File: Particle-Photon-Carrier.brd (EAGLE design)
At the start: 46 x 35.3 mm, 44 parts, among them J2 5V @ 2A, Q1 BSS138, Q2 BSS138, Q3 BSS138, Q4 BSS138

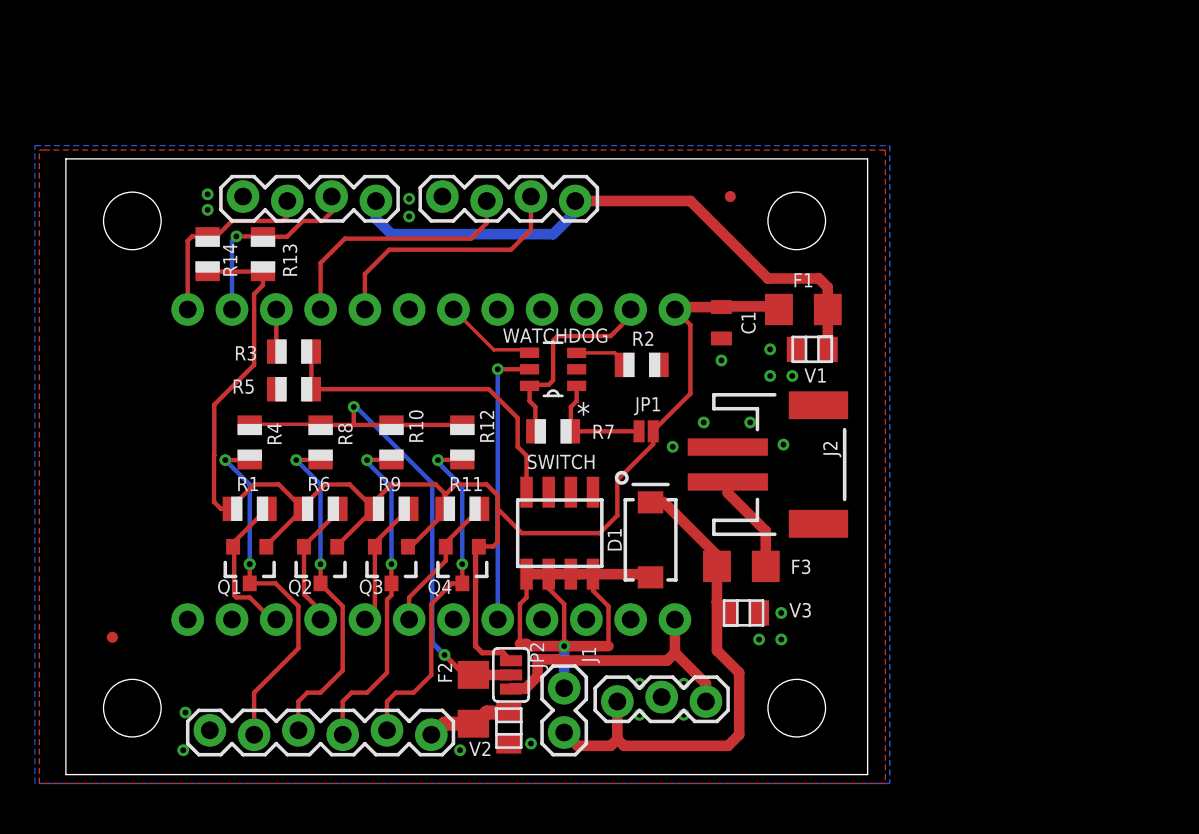
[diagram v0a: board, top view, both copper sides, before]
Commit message: v3 of the AquaMaster
For Spring 2018
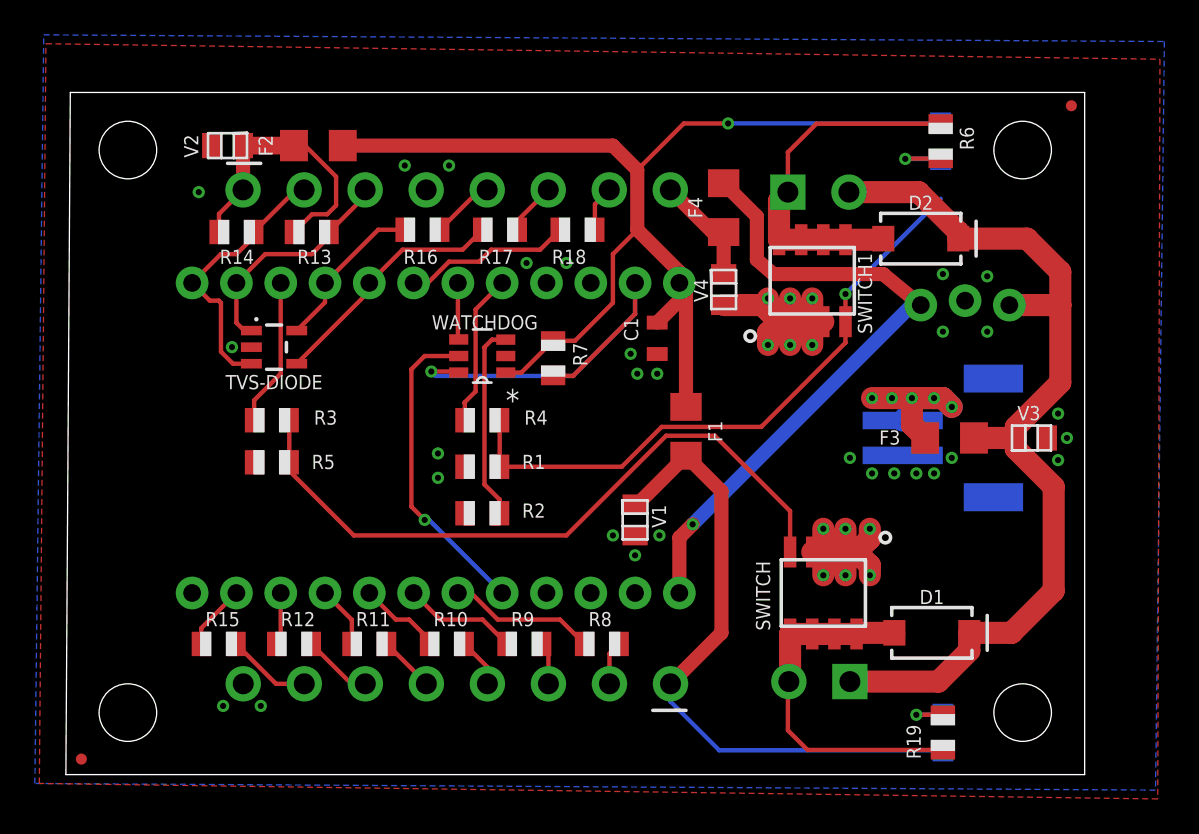
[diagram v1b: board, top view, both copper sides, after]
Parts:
- removed 12V-5V-BUCK: I50115, SparkFun-Connectors:1X03_LOCK
- removed D-IO, I2C: (no value), SparkFun-Connectors:1X04_LOCK
- removed JP1: DOG-SW, SparkFun-Jumpers:SMT-JUMPER_2_NO_NO-SILK
- removed JP2: VSelect, SparkFun-Jumpers:SMT-JUMPER_3_1-NC_PASTE_SILK
- removed Q1, Q2, Q3, Q4: BSS138, SparkFun:SOT23-3
- removed SPI: (no value), SparkFun-Connectors:1X06_LOCK
- added ANALOG, DIGITAL: (no value), SparkFun-Connectors:SCREWTERMINAL-3.5MM-8
- added D2: 3A/40V/500mV, SparkFun-DiscreteSemi:SMA-DIODE
- added F4: 500mA - FAST BLOW, SparkFun-Fuses:1206
- added J3: (no value), SparkFun-Connectors:1X03_LOCK
- added J4: (no value), SparkFun-Connectors:SCREWTERMINAL-3.5MM-2
- added LED1, LED2: (no value), adafruit:CHIPLED_0805
- added R15, R16, R17, R18, R19: 1k, adafruit:R0805
- added SWITCH1: IRF6201PBF, MOSFETs:SO8-GW300
- added TVS-DIODE: D5V0L4B5TS, Custom Components:SOT-23-5
- added V4: VC080505C150DP, Custom Components:0805
- J1: device SparkFun-Connectors:1X02 -> SparkFun-Connectors:SCREWTERMINAL-3.5MM-2
- R1: value 10K -> 100k
- R10, R11, R12, R4, R6, R8, R9: value 10K -> 1k
- moved R6 41.3 mm to (50.2, 36.3), turned to 90 degrees
- moved V2 37.1 mm to (9.27, 36.1), turned to 0 degrees
- moved F2 33.0 mm to (14.5, 36.1), turned to 180 degrees
- moved FD2 20.2 mm to (57.7, 38.4)
- moved R8 19.8 mm to (30.7, 7.49), turned to 0 degrees
- moved V3 19.3 mm to (55.4, 19.3)
- moved D1 17.0 mm to (49.7, 8.13), turned to 0 degrees
- moved J1 16.4 mm to (45.0, 5.33), flipped to the bottom, turned to 0 degrees
- moved SWITCH 15.5 mm to (43.4, 10.4)
- moved R12 15.1 mm to (13.1, 7.49), turned to 0 degrees
- moved V1 14.1 mm to (32.6, 14.6), turned to 90 degrees
- moved F3 14.0 mm to (50.7, 19.3), turned to 0 degrees
- moved JP5 13.6 mm to (54.9, 35.8)
- moved R1 13.6 mm to (23.9, 17.7)
- moved R4 13.4 mm to (23.9, 20.3), turned to 0 degrees
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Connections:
- net SOLENOID renamed SOLENOID1
- removed net A2-EXT: Q1.3, R4.2, SPI.2
- removed net A3-EXT: Q2.3, R8.2, SPI.3
- removed net A4-EXT: Q3.3, R10.2, SPI.4
- removed net A5-EXT: Q4.3, R12.2, SPI.5
- removed net VCC-EXT: D-IO.4, F1.2, I2C.4, V1.2
- removed net VIO-EXT: F2.2, SPI.6, V2.2
- removed net VSELECT: F2.1, JP2.2, R10.1, R12.1, R4.1, R8.1
- new net A0: PHOTON.12
- new net A1: PHOTON.11, R15.1
- new net D5: PHOTON.18, R18.1
- new net DAC: PHOTON.6, R8.1
- new net EXT-A1: ANALOG.7, R15.2
- new net EXT-A2: ANALOG.6, R12.2
- new net EXT-A3: ANALOG.5, R11.2
- new net EXT-A4: ANALOG.4, R10.2
- new net EXT-A5: ANALOG.3, R9.2
- new net EXT-D3: DIGITAL.5, R16.2
- new net EXT-D4: DIGITAL.6, R17.2
- new net EXT-D5: DIGITAL.7, R18.2
- new net EXT-DAC: ANALOG.2, R8.2
- new net GATE1: R1.2, R4.2, SWITCH1.4
- new net LOAD-GND2: D2.A, J4.1, R6.2, SWITCH1.5, SWITCH1.6, SWITCH1.7, SWITCH1.8
- new net N$2: LED1.C, R19.2
- new net RX: PHOTON.4
- new net SOLENOID2: PHOTON.20, R4.1
- new net TX: PHOTON.3
- new net VCC1-EXT: ANALOG.1, F1.2, LED1.A, V1.2
- new net VCC2-EXT: DIGITAL.1, F2.2, R13.2, R14.2, V2.2
- new net VIN-EXT: DIGITAL.8, F4.2, V4.2
- net A2: now also R12.1; no longer Q1.2, R1.2
- net A3: now also R11.1; no longer Q2.2, R6.2
- net A4: now also R10.1; no longer Q3.2, R9.2
- net A5: now also R9.1; no longer Q4.2, R11.2
- net D3: now also R16.1, TVS-DIODE.5; no longer D-IO.2
- net D4: now also R17.1, TVS-DIODE.4; no longer D-IO.3
- net DC-IN: now also D2.C, J1.1, J3.3, J4.2; no longer 12V-5V-BUCK.3, J1.2
- net GND: now also ANALOG.8, DIGITAL.4, J3.2, R1.1, SWITCH1.1, SWITCH1.2, SWITCH1.3, TVS-DIODE.2, V4.1; no longer 12V-5V-BUCK.2, D-IO.1, I2C.1, SPI.1
- net LOAD-GND: now also J1.2, R19.1; no longer J1.1
- net N$1: now also LED2.C, R6.1; no longer JP1.1, R7.1, WATCHDOG.1
- net SCL: now also DIGITAL.3, TVS-DIODE.1; no longer I2C.3
- net SDA: now also DIGITAL.2, TVS-DIODE.3; no longer I2C.2
- net VCC: now also F2.1, LED2.A, R7.1, WATCHDOG.1; no longer JP1.2, JP2.3, Q1.1, Q2.1, Q3.1, Q4.1, R1.1, R11.1, R13.2, R14.2, R6.1, R9.1
- net VIN: now also F4.1, J3.1; no longer 12V-5V-BUCK.1, JP2.1
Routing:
- net VCC1-EXT: track 0.00 -> 37.0 mm
- net GATE1: track 0.00 -> 36.0 mm, vias 0 -> 1
- net VCC-EXT: track 34.1 -> 0.00 mm
- net VSELECT: track 34.0 -> 0.00 mm, vias 2 -> 0
- net GND: track 0.00 -> 26.2 mm, vias 23 -> 41
- net DC-IN: track 29.9 -> 54.6 mm
- net VCC: track 89.1 -> 66.3 mm, vias 0 -> 1
- net VIN: track 16.3 -> 38.1 mm, vias 0 -> 1
- net A2-EXT: track 20.8 -> 0.00 mm, vias 2 -> 0
- net LOAD-GND2: track 0.00 -> 20.7 mm
- net GATE: track 19.1 -> 39.7 mm
- net A5-EXT: track 20.2 -> 0.00 mm, vias 2 -> 0
- net A3-EXT: track 19.5 -> 0.00 mm, vias 2 -> 0
- net A4-EXT: track 19.4 -> 0.00 mm, vias 2 -> 0
- net VCC2-EXT: track 0.00 -> 16.3 mm
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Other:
- board size 46 x 35.3 mm -> 58.4 x 39.1 mm
- board text added: "12V @3A +"
- board text added: "GND Load2"
- board text added: "Load1 GND"
- board text added: "VCC DAC A5 A4 A3 A2 A1 GND"
- board text added: "VOUT GND VIN"
- board text added: "Vcc SDA SCL GND D3 D4 D5 Vin"
- board text added: "chip@seeinsights.com 04-11-18 Photon Carrier v3"
- board text removed: "LOAD"
- board text removed: "OUT GND IN"
- board text removed: "VCC A5 A4 A3 A2 GND"
- board text removed: "VCC D4 D3 GND"
- board text removed: "chip@seeinsights.com 8-22-17 Photon Carrier v2"
